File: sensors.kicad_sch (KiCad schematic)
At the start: 6 parts, among them U10 TMP235, U11 ACS723xLCTR-05AB

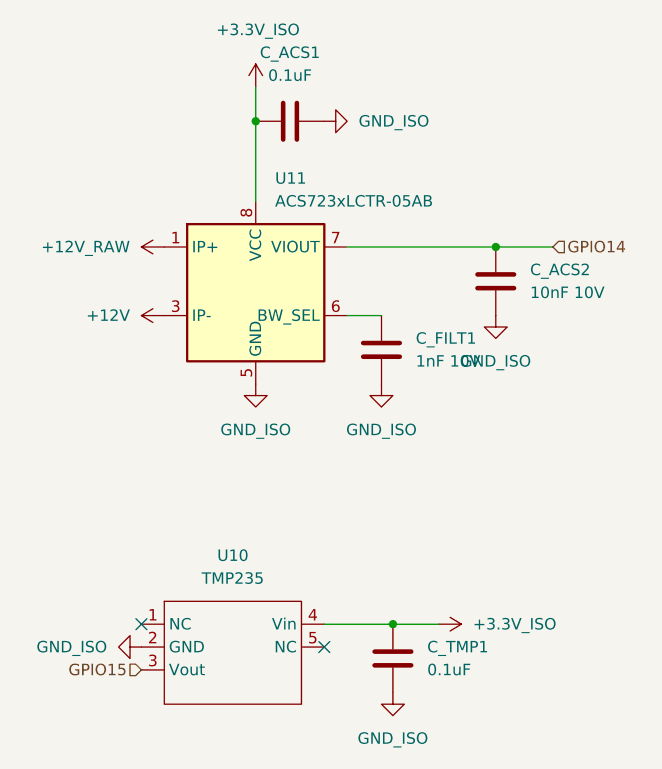
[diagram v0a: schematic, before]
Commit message: V 1.2
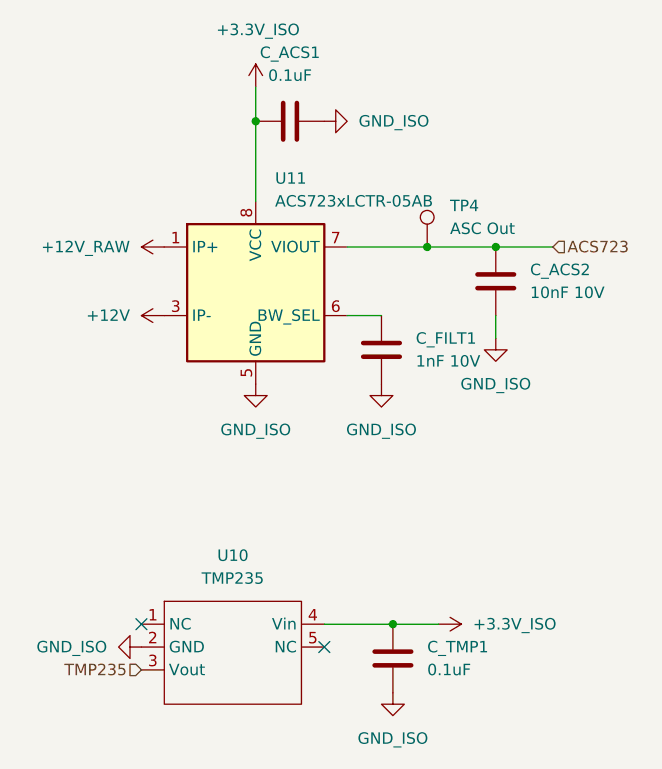
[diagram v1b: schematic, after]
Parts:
- added TP4: ASC Out, barn_shade_controller:TestPoint_Pad_D1.0mm_No_SolderMask, symbol Connector:TestPoint
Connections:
- net GPIO14 renamed ACS723
- net ACS723: now also TP4.1
- net GPIO15 renamed TMP235
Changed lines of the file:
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@@
+		(color 0 0 0 0)
+	)
+	(junction
+		(at 102.87 43.18)
+		(diameter 0)
 		(color 0 0 0 0)
 	)
@@
 	(no_connect
 		(at 71.12 85.09)
+	)
+	(wire
+		(pts
+			(xy 110.49 53.34) (xy 110.49 50.8)
+		)
+		(stroke
+			(width 0)
+			(type default)
+		)
 	)
 	(wire
@@
 	(wire
 		(pts
-			(xy 110.49 43.18) (xy 93.98 43.18)
+			(xy 110.49 43.18) (xy 102.87 43.18)
 		)
 		(stroke
@@
 	(wire
 		(pts
-			(xy 83.82 25.4) (xy 83.82 29.21)
+			(xy 102.87 43.18) (xy 93.98 43.18)
 		)
 		(stroke
@@
 	(wire
 		(pts
-			(xy 99.06 85.09) (xy 91.44 85.09)
+			(xy 83.82 25.4) (xy 83.82 29.21)
 		)
 		(stroke
@@
 	(wire
 		(pts
-			(xy 97.79 50.8) (xy 93.98 50.8)
+			(xy 99.06 85.09) (xy 91.44 85.09)
 		)
 		(stroke
@@
 	(wire
 		(pts
-			(xy 116.84 43.18) (xy 110.49 43.18)
+			(xy 97.79 50.8) (xy 93.98 50.8)
 		)
 		(stroke
@@
 		)
 	)
-	(hierarchical_label "GPIO15"
+	(wire
+		(pts
+			(xy 116.84 43.18) (xy 110.49 43.18)
+		)
+		(stroke
+			(width 0)
+			(type default)
+		)
+	)
+	(hierarchical_label "TMP235"
 		(shape input)
 		(at 71.12 90.17 180)
@@
 		)
 	)
-	(hierarchical_label "GPIO14"
+	(hierarchical_label "ACS723"
 		(shape input)
 		(at 116.84 43.18 0)
@@
 	(symbol
 		(lib_id "power:GND")
-		(at 110.49 50.8 0)
+		(at 110.49 53.34 0)
 		(unit 1)
 		(exclude_from_sim no)
@@
 		(fields_autoplaced yes)
 		(property "Reference" "#PWR087"
-			(at 110.49 57.15 0)
+			(at 110.49 59.69 0)
 			(effects
 				(font
@@
 		)
 		(property "Value" "GND_ISO"
-			(at 110.49 55.88 0)
+			(at 110.49 58.42 0)
 			(effects
 				(font
@@
 		)
 		(property "Footprint" ""
-			(at 110.49 50.8 0)
+			(at 110.49 53.34 0)
 			(effects
 				(font
@@
 		)
 		(property "Datasheet" ""
-			(at 110.49 50.8 0)
+			(at 110.49 53.34 0)
 			(effects
 				(font
@@
 		)
 		(property "Description" "Power symbol creates a global label with name \"GND\" , ground"
-			(at 110.49 50.8 0)
+			(at 110.49 53.34 0)
 			(effects
 				(font
@@
 					(unit 1)
 				)
+			)
+		)
+	)
+	(symbol
+		(lib_id "Connector:TestPoint")
+		(at 102.87 43.18 0)
+		(unit 1)
+		(exclude_from_sim no)
+		(in_bom yes)
+		(on_board yes)
+		(dnp no)
+		(fields_autoplaced yes)
+		(property "Reference" "TP4"
+			(at 105.41 38.6079 0)
+			(effects
+				(font
+					(size 1.27 1.27)
+				)
+				(justify left)
+			)
+		)
+		(property "Value" "ASC Out"
+			(at 105.41 41.1479 0)
+			(effects
+				(font
+					(size 1.27 1.27)
+				)
+				(justify left)
+			)
+		)
+		(property "Footprint" "barn_shade_controller:TestPoint_Pad_D1.0mm_No_SolderMask"
+			(at 107.95 43.18 0)
+			(effects
+				(font
+					(size 1.27 1.27)
+				)
+				(hide yes)
+			)
+		)
+		(property "Datasheet" "~"
+			(at 107.95 43.18 0)
+			(effects
+				(font
+					(size 1.27 1.27)
+				)
+				(hide yes)
+			)
+		)
+		(property "Description" "test point"
+			(at 102.87 43.18 0)
+			(effects
+				(font
+					(size 1.27 1.27)
+				)
+				(hide yes)
+			)
+		)
+		(pin "1"
+		)
+		(instances
+			(project "barn-blinds-controller"
+				(path "/aa90962a-81b9-423d-8acd-c4e83fa798bb/8f0cb6d8-027e-4edb-b8ea-04d7ddb83db1"
+					(reference "TP4")
+					(unit 1)
+				)
